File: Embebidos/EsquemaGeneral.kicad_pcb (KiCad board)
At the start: 2 copper layers, 100 x 99.9 mm, 79 parts, among them IC1 ESP32-WROVER-B__8MB_, J1 USB_A, J2 Conn_01x02, J3 RJ45, J4 RJ45, J5 Conn_02x06_Counter_Clockwise, J6 Conn_01x08, J7 Conn_01x04, Q1 BC847, Q2 BC847, Q3 BSS138, Q4 DMP3056LSDQ-13, Q5 BSS138, Q6 DMP3056LSDQ-13, SW1 SW_Reset, SW2 SW_Boot, U2 LM358, U3 SPX3819M5-L-3-3, U4 MIC29302WU, U5 MIC5219-3.3YM5

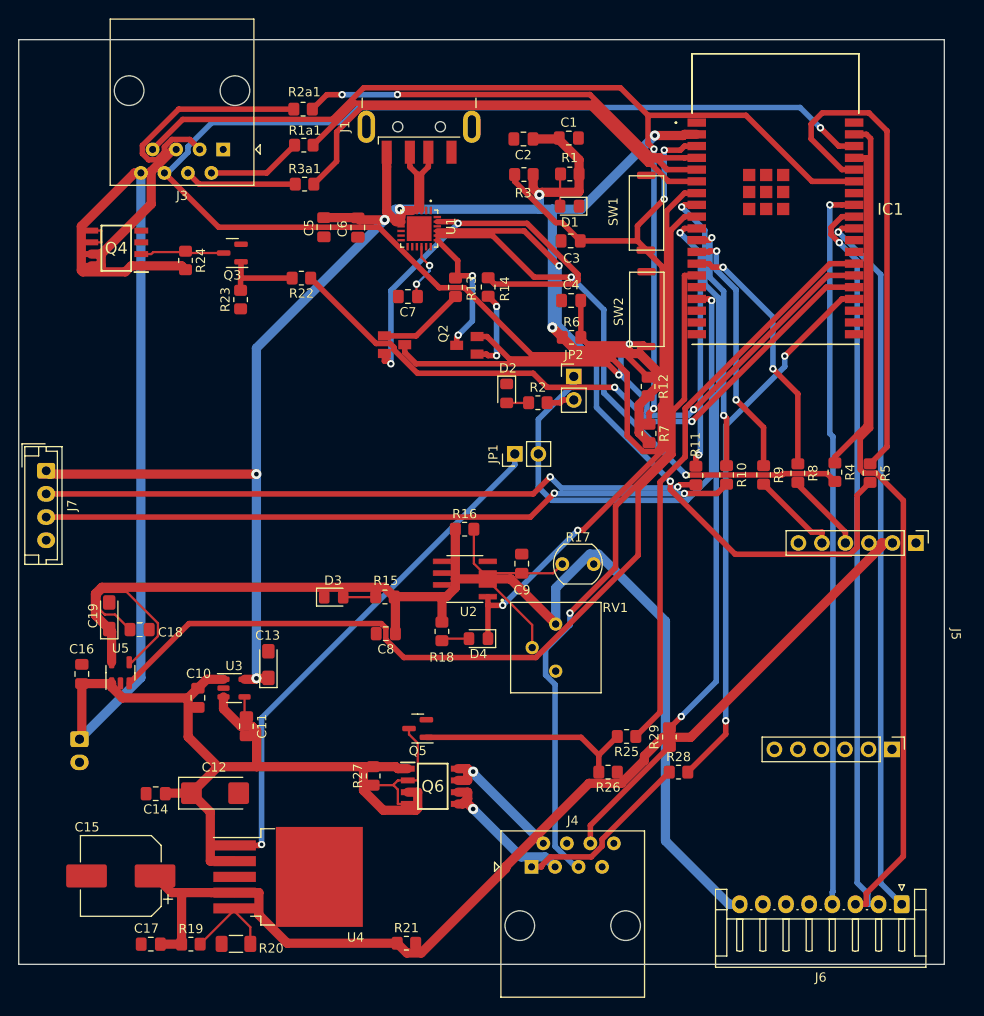
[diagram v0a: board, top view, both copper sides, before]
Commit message: eliminar pistas para volver a intetar
:c
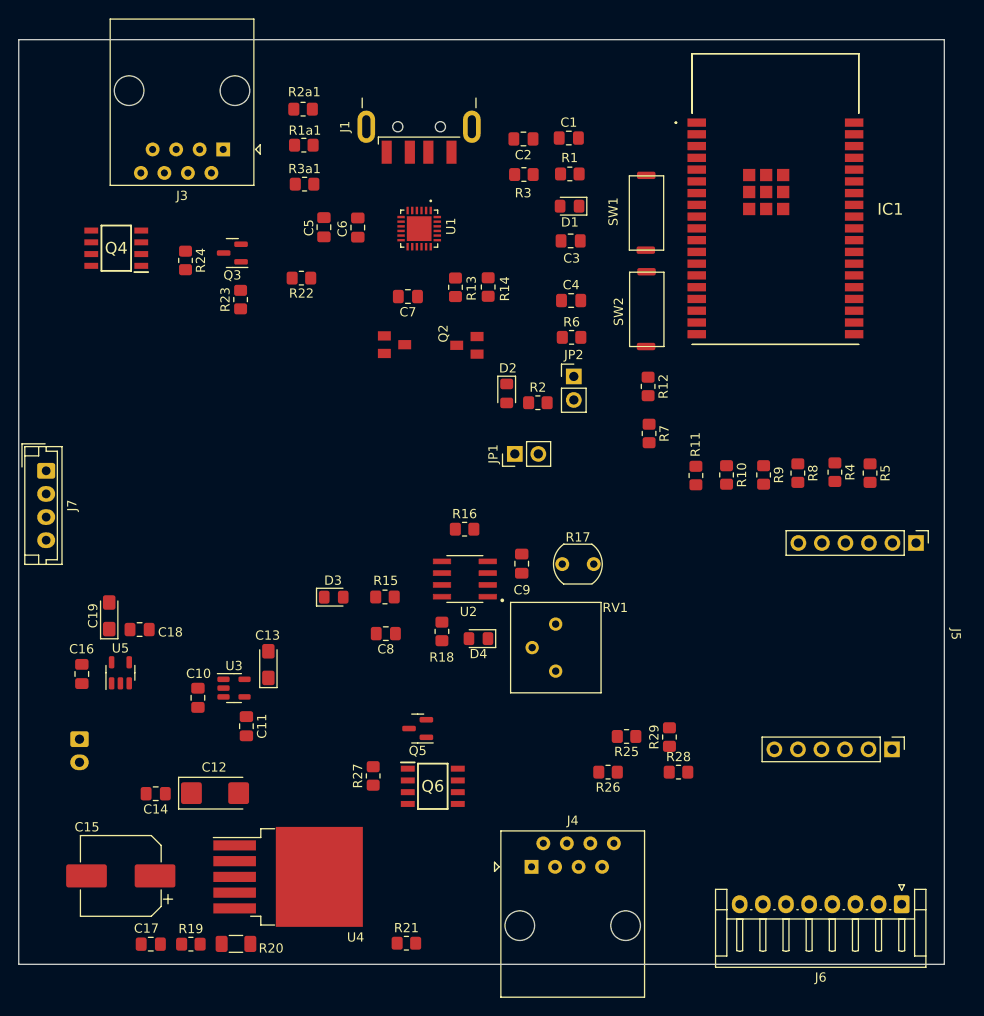
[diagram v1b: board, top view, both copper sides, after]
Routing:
- net +3.3V: track 1452.3 -> 0.00 mm, vias 27 -> 0
- net 4.1V: track 322.6 -> 0.00 mm, vias 8 -> 0
- net 3.3Vop2: track 174.8 -> 0.00 mm
- net Net-(IC1-Pad35): track 126.3 -> 0.00 mm
- net /Acondicionamiento/SCK_RFID: track 78.9 -> 0.00 mm, vias 1 -> 0
- net /Acondicionamiento/MISO_RFID: track 78.3 -> 0.00 mm, vias 1 -> 0
- net /Acondicionamiento/CS_RFID: track 77.3 -> 0.00 mm, vias 1 -> 0
- net /Acondicionamiento/RXGPS: track 75.0 -> 0.00 mm, vias 2 -> 0
- net /Acondicionamiento/TXGPS: track 71.6 -> 0.00 mm, vias 2 -> 0
- net /Acondicionamiento/ctr_led_delantero: track 71.3 -> 0.00 mm, vias 2 -> 0
- net /Acondicionamiento/ctr_trasero: track 62.4 -> 0.00 mm
- net /Acondicionamiento/Din_der: track 59.3 -> 0.00 mm, vias 2 -> 0
- net Net-(IC1-Pad34): track 53.8 -> 0.00 mm
- net /USB_UART/DTR: track 48.2 -> 0.00 mm, vias 2 -> 0
- net /Luces traseras/VCC_INF: track 35.3 -> 0.00 mm, vias 1 -> 0
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
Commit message: siiiiiiiiii
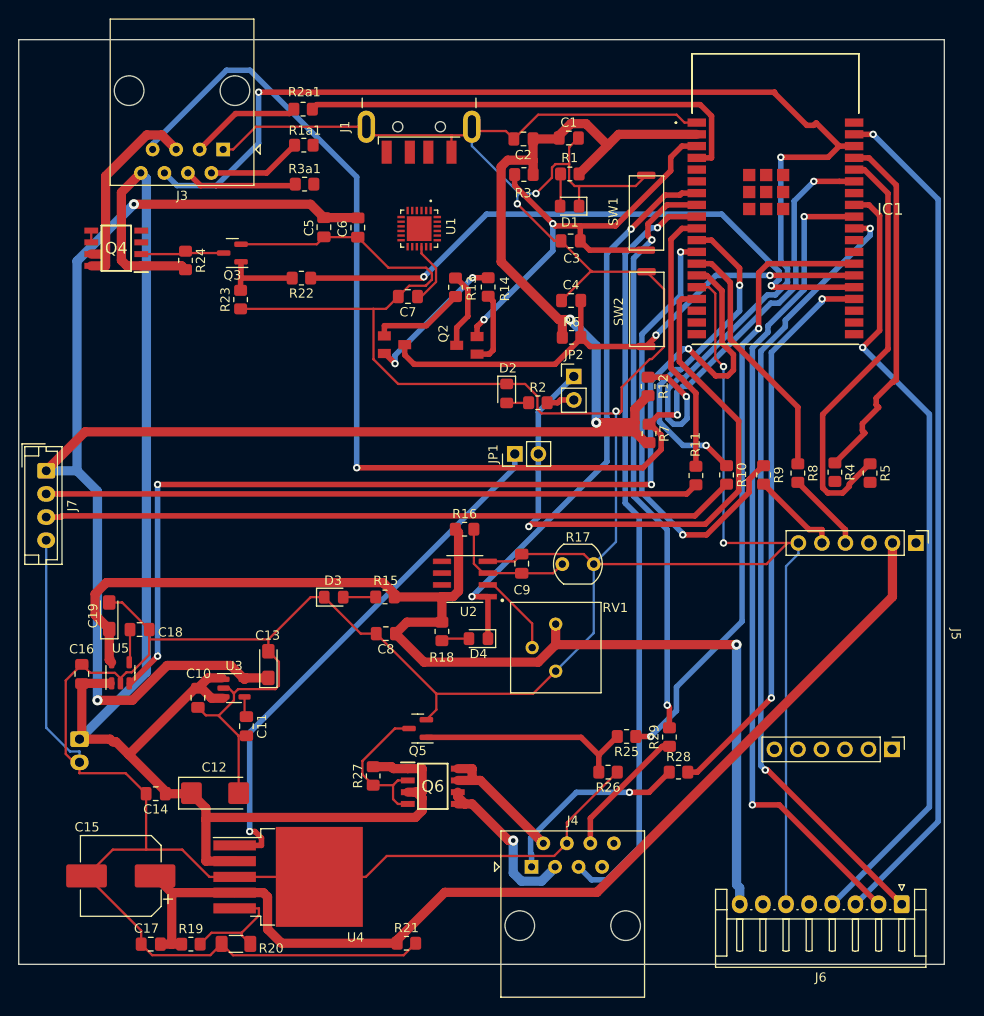
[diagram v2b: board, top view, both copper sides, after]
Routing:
- net GND: track 0.00 -> 615.0 mm, vias 0 -> 5
- net +3.3V: track 0.00 -> 248.4 mm, vias 0 -> 4
- net +5V: track 0.00 -> 169.7 mm
- net /Acondicionamiento/SDA_PAN: track 0.00 -> 139.4 mm, vias 0 -> 3
- net /Acondicionamiento/SCL_PAN: track 0.00 -> 136.7 mm, vias 0 -> 3
- net 3.3Vop2: track 0.00 -> 133.4 mm, vias 0 -> 1
- net 4.1V: track 0.00 -> 114.1 mm
- net CtrlOnOff: track 0.00 -> 111.7 mm, vias 0 -> 4
- net /Acondicionamiento/MOSI_RFID: track 0.00 -> 91.8 mm, vias 0 -> 1
- net /Acondicionamiento/SCK_RFID: track 0.00 -> 89.3 mm, vias 0 -> 2
- net /Acondicionamiento/CS_RFID: track 0.00 -> 86.1 mm, vias 0 -> 2
- net /Acondicionamiento/MISO_RFID: track 0.00 -> 85.7 mm, vias 0 -> 1
- net /Acondicionamiento/VO_Inf: track 0.00 -> 82.7 mm, vias 0 -> 1
- net /Acondicionamiento/RXGPS: track 0.00 -> 75.0 mm
- net /Acondicionamiento/TXGPS: track 0.00 -> 70.6 mm
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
